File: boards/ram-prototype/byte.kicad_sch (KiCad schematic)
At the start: 48 parts, among them U1 74LVC1G79, U10 74LVC1G125, U11 74LVC1G79, U12 74LVC1G125, U13 74LVC1G79, U14 74LVC1G125, U15 74LVC1G79, U16 74LVC1G125, U2 74LVC1G125, U3 74LVC1G79, U4 74LVC1G125, U5 74LVC1G79, U6 74LVC1G125, U7 74LVC1G79, U8 74LVC1G125, U9 74LVC1G79

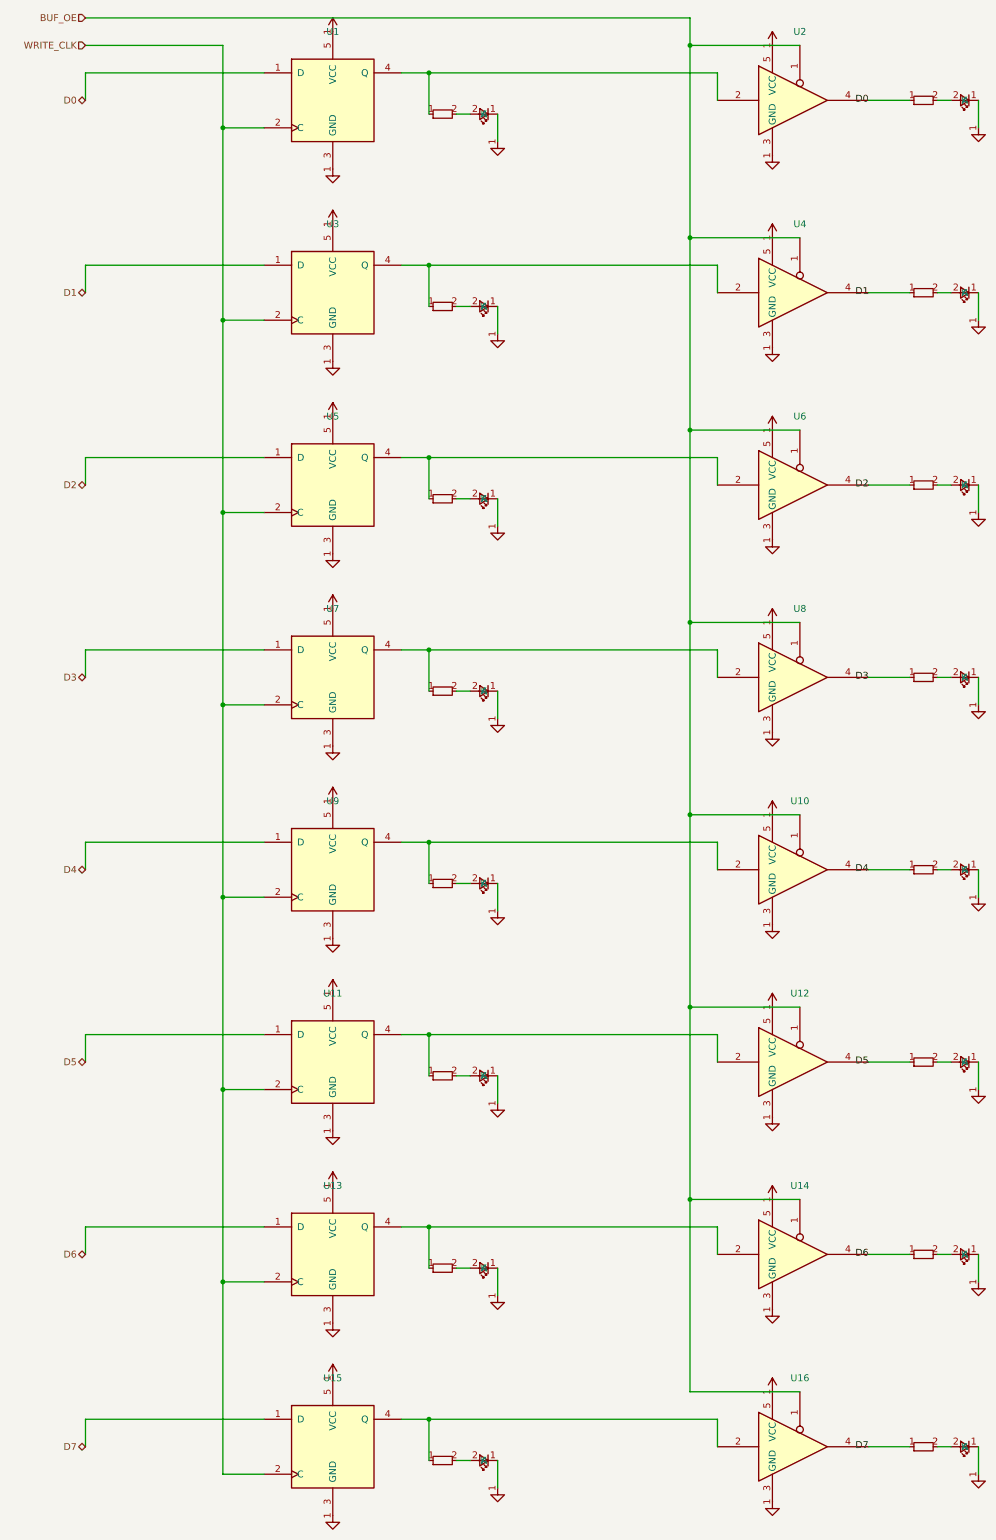
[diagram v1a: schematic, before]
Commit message: Clean up root
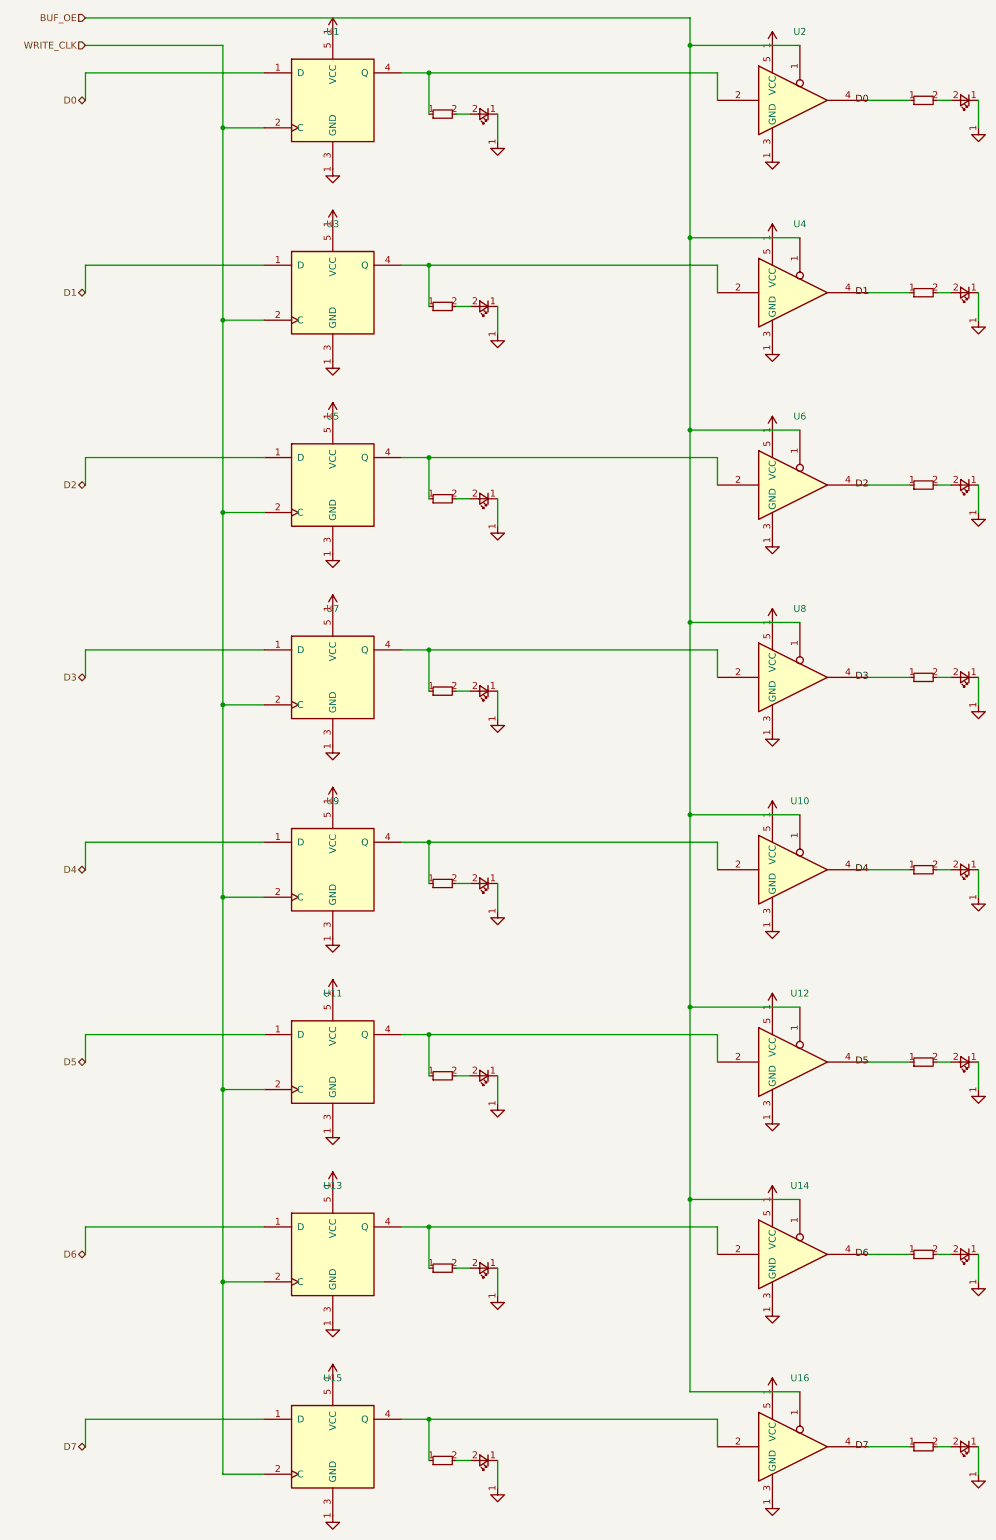
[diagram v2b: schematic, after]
